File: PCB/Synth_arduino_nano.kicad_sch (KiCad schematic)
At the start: 20 parts, among them J1 FSLP, SW1 RECSW, U1 DM-OLED096-636

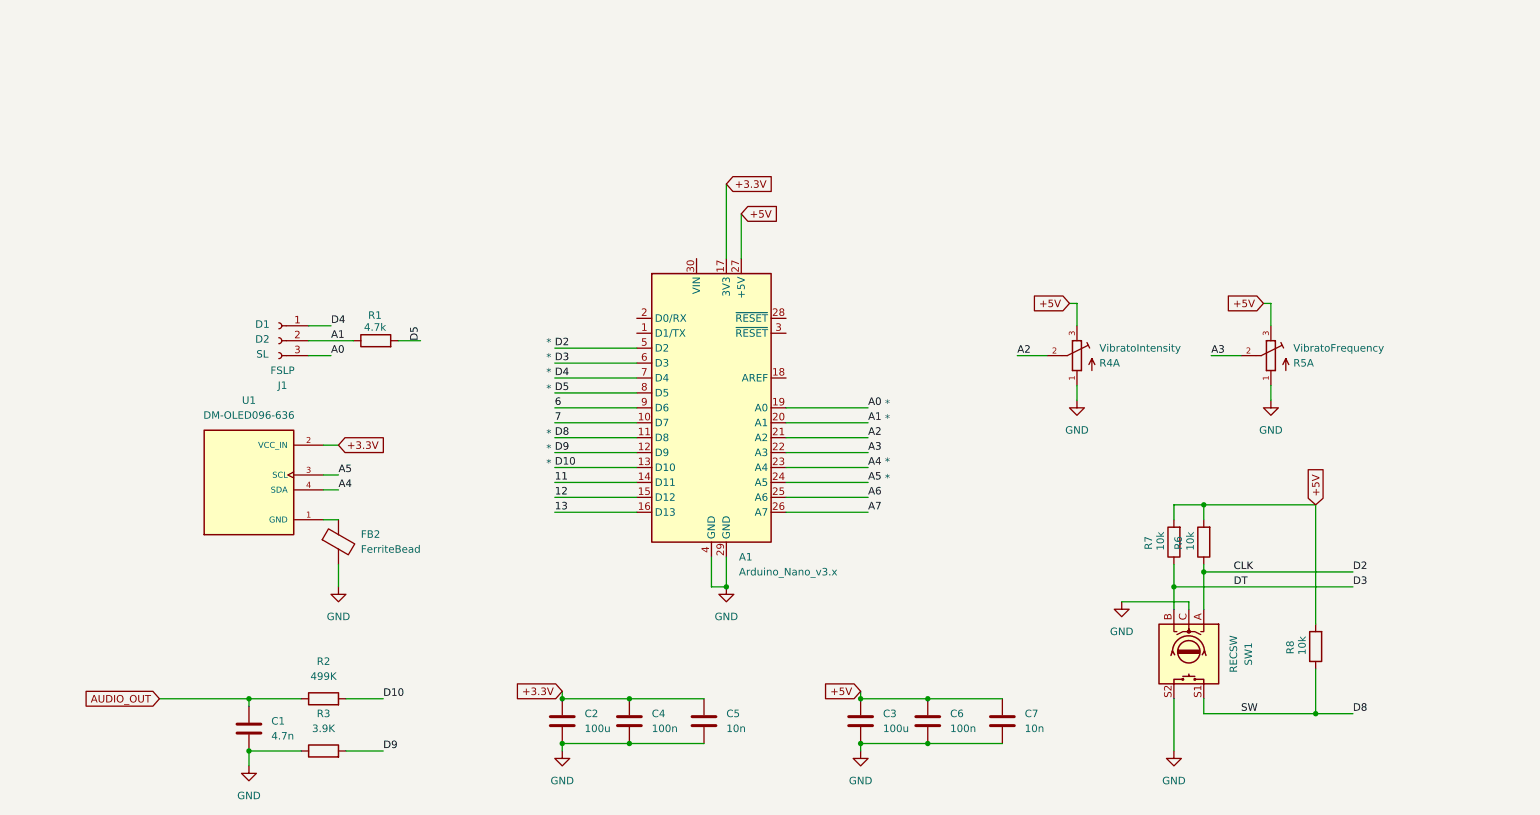
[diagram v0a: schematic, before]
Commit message: Add files via upload
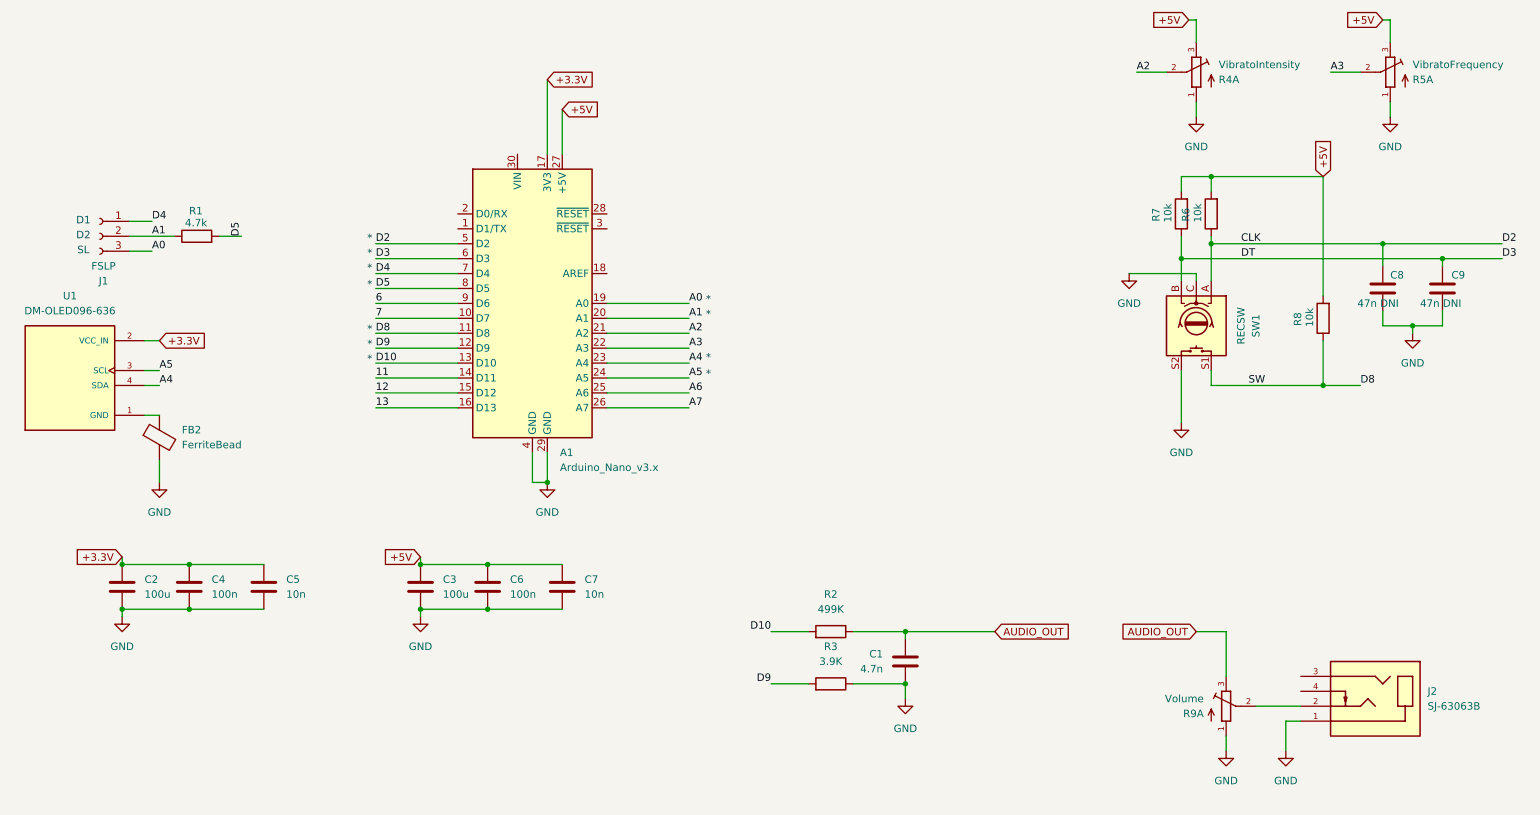
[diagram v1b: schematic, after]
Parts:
- added C8, C9: 47n DNI, Capacitor_SMD:C_0603_1608Metric_Pad1.08x0.95mm_HandSolder, symbol Device:C
- added J2: SJ-63063B, SJ63063B:CUI_SJ-63063B, symbol SJ63063B:SJ-63063B
- added R9: Volume, PTV09A:PTV09A-4025F-B103, symbol PTV09A:PTV09A-4025F-B103
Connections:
- net AUDIO_OUT: now also R9.3
- net CLK: now also C8.1
- net D3: now also C9.1
- net GND: now also C8.2, C9.2, J2.1, R9.1
- new net: J2.2, R9.2
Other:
- moved on the sheet: A1, C1, C2, C3, C4, C5, C6, C7, FB2, J1, R1, R2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
